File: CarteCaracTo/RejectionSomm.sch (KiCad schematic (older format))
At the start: 6 parts, among them U1 OPA4376

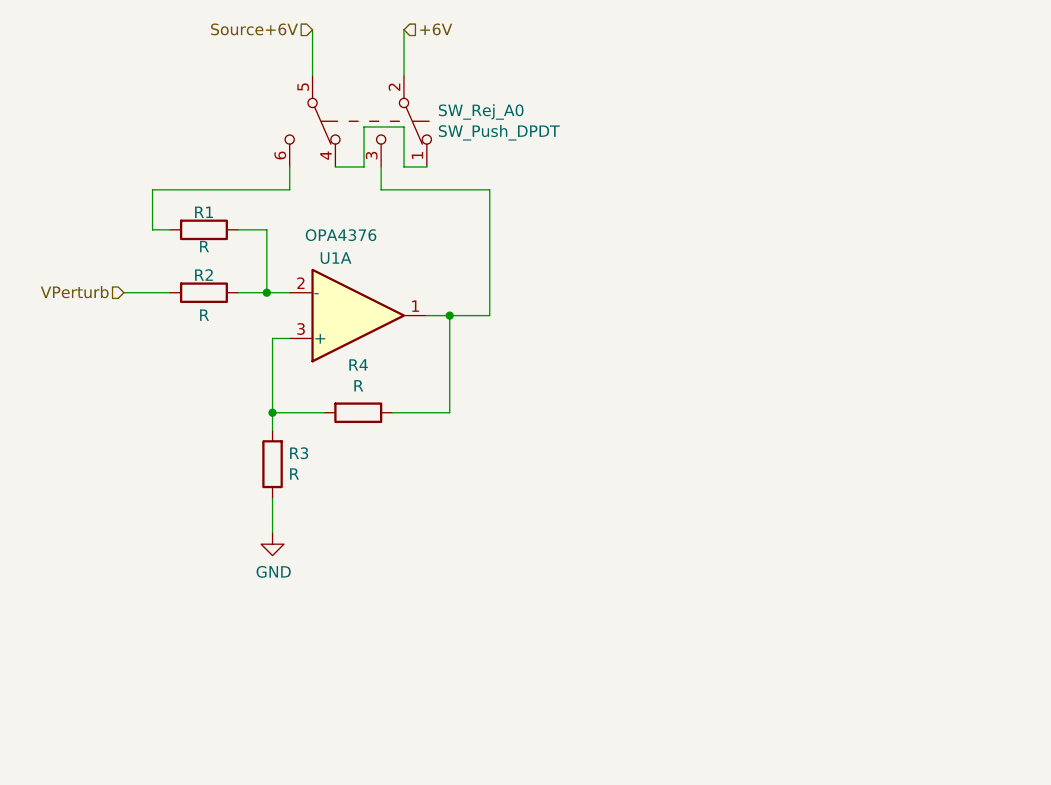
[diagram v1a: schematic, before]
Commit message: Routé, verif pre-envoie
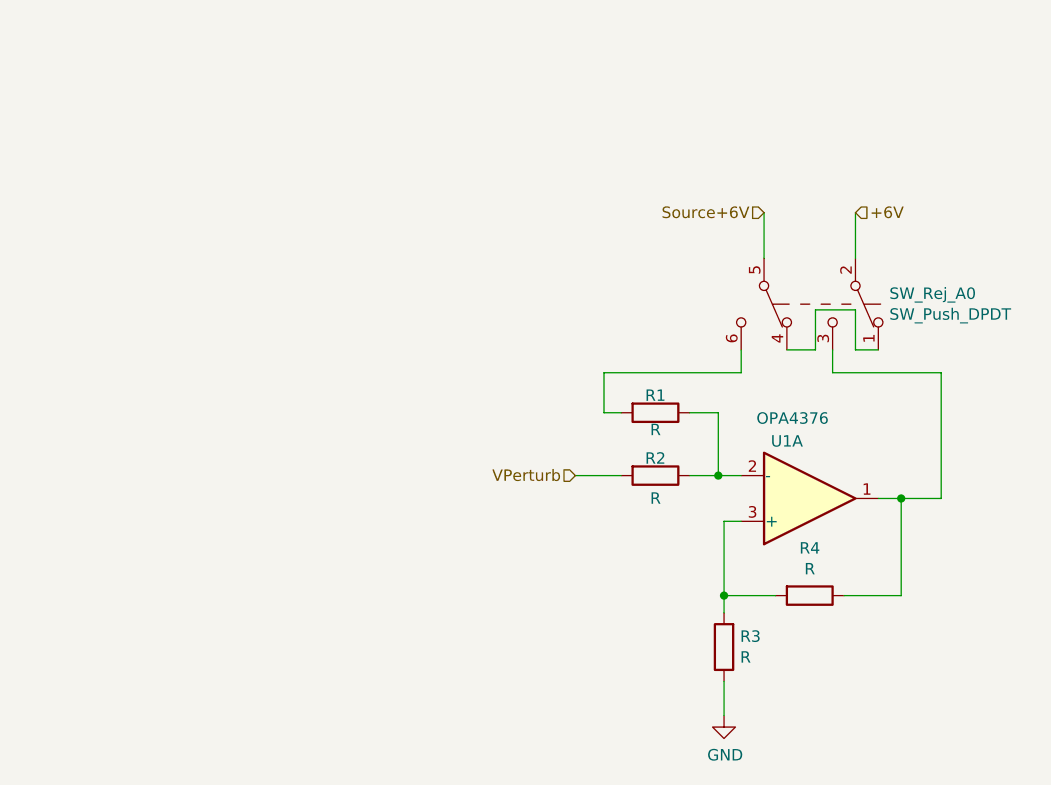
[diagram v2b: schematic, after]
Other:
- moved on the sheet: R1, R2, R3, R4, SW_Rej_A0, U1A
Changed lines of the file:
@@
 $Descr A4 11693 8268
 encoding utf-8
-Sheet 121 122
+Sheet 120 122
 Title ""
 Date ""
@@
 L Amplifier_Operational:OPA4376 U?
 U 1 1 61D78C60
-P 3450 3075
+P 5425 3875
 AR Path="/61D78C60" Ref="U?"  Part="1"
 AR Path="/61D6BED7/61D78C60" Ref="U1"  Part="1"
 AR Path="/61F56081/61D78C60" Ref="U1"  Part="2"
 AR Path="/61F9BC15/61D78C60" Ref="U1"  Part="3"
-F 0 "U1" H 3350 2825 50  0000 C CNN
-F 1 "OPA4376" H 3375 2725 50  0000 C CNN
-F 2 "Package_SO:SOIC-14_3.9x8.7mm_P1.27mm" H 3400 3175 50  0001 C CNN
-F 3 "http://www.ti.com/lit/ds/symlink/opa376.pdf" H 3500 3275 50  0001 C CNN
-	1    3450 3075
+F 0 "U1" H 5325 3625 50  0000 C CNN
+F 1 "OPA4376" H 5350 3525 50  0000 C CNN
+F 2 "Package_SO:SOIC-14_3.9x8.7mm_P1.27mm" H 5375 3975 50  0001 C CNN
+F 3 "http://www.ti.com/lit/ds/symlink/opa376.pdf" H 5475 4075 50  0001 C CNN
+	1    5425 3875
 	1    0    0    1
 $EndComp
@@
 L Device:R R?
 U 1 1 61D78C66
-P 2775 2700
+P 4750 3500
 AR Path="/61D78C66" Ref="R?"  Part="1"
 AR Path="/61D6BED7/61D78C66" Ref="R1"  Part="1"
 AR Path="/61F56081/61D78C66" Ref="R5"  Part="1"
 AR Path="/61F9BC15/61D78C66" Ref="R9"  Part="1"
-F 0 "R1" V 2700 2700 50  0000 C CNN
-F 1 "R" V 2850 2700 50  0000 C CNN
-F 2 "Resistor_SMD:R_0603_1608Metric_Pad1.05x0.95mm_HandSolder" V 2705 2700 50  0001 C CNN
-F 3 "~" H 2775 2700 50  0001 C CNN
-	1    2775 2700
+F 0 "R1" V 4675 3500 50  0000 C CNN
+F 1 "R" V 4825 3500 50  0000 C CNN
+F 2 "Resistor_SMD:R_0603_1608Metric_Pad1.05x0.95mm_HandSolder" V 4680 3500 50  0001 C CNN
+F 3 "~" H 4750 3500 50  0001 C CNN
+	1    4750 3500
 	0    1    1    0
 $EndComp
@@
 L Device:R R?
 U 1 1 61D78C6C
-P 2775 2975
+P 4750 3775
 AR Path="/61D78C6C" Ref="R?"  Part="1"
 AR Path="/61D6BED7/61D78C6C" Ref="R2"  Part="1"
 AR Path="/61F56081/61D78C6C" Ref="R6"  Part="1"
 AR Path="/61F9BC15/61D78C6C" Ref="R10"  Part="1"
-F 0 "R2" V 2700 2975 50  0000 C CNN
-F 1 "R" V 2875 2975 50  0000 C CNN
-F 2 "Resistor_SMD:R_0603_1608Metric_Pad1.05x0.95mm_HandSolder" V 2705 2975 50  0001 C CNN
-F 3 "~" H 2775 2975 50  0001 C CNN
-	1    2775 2975
+F 0 "R2" V 4675 3775 50  0000 C CNN
+F 1 "R" V 4850 3775 50  0000 C CNN
+F 2 "Resistor_SMD:R_0603_1608Metric_Pad1.05x0.95mm_HandSolder" V 4680 3775 50  0001 C CNN
+F 3 "~" H 4750 3775 50  0001 C CNN
+	1    4750 3775
 	0    1    1    0
 $EndComp
@@
 L Device:R R?
 U 1 1 61D78C72
-P 3075 3725
+P 5050 4525
 AR Path="/61D78C72" Ref="R?"  Part="1"
 AR Path="/61D6BED7/61D78C72" Ref="R3"  Part="1"
 AR Path="/61F56081/61D78C72" Ref="R7"  Part="1"
 AR Path="/61F9BC15/61D78C72" Ref="R11"  Part="1"
-F 0 "R3" H 3005 3679 50  0000 R CNN
-F 1 "R" H 3005 3770 50  0000 R CNN
-F 2 "Resistor_SMD:R_0603_1608Metric_Pad1.05x0.95mm_HandSolder" V 3005 3725 50  0001 C CNN
-F 3 "~" H 3075 3725 50  0001 C CNN
-	1    3075 3725
+F 0 "R3" H 4980 4479 50  0000 R CNN
+F 1 "R" H 4980 4570 50  0000 R CNN
+F 2 "Resistor_SMD:R_0603_1608Metric_Pad1.05x0.95mm_HandSolder" V 4980 4525 50  0001 C CNN
+F 3 "~" H 5050 4525 50  0001 C CNN
+	1    5050 4525
 	-1   0    0    1
 $EndComp
@@
 L Device:R R?
 U 1 1 61D78C78
-P 3450 3500
+P 5425 4300
 AR Path="/61D78C78" Ref="R?"  Part="1"
 AR Path="/61D6BED7/61D78C78" Ref="R4"  Part="1"
 AR Path="/61F56081/61D78C78" Ref="R8"  Part="1"
 AR Path="/61F9BC15/61D78C78" Ref="R12"  Part="1"
-F 0 "R4" V 3243 3500 50  0000 C CNN
-F 1 "R" V 3334 3500 50  0000 C CNN
-F 2 "Resistor_SMD:R_0603_1608Metric_Pad1.05x0.95mm_HandSolder" V 3380 3500 50  0001 C CNN
-F 3 "~" H 3450 3500 50  0001 C CNN
-	1    3450 3500
+F 0 "R4" V 5218 4300 50  0000 C CNN
+F 1 "R" V 5309 4300 50  0000 C CNN
+F 2 "Resistor_SMD:R_0603_1608Metric_Pad1.05x0.95mm_HandSolder" V 5355 4300 50  0001 C CNN
+F 3 "~" H 5425 4300 50  0001 C CNN
+	1    5425 4300
 	0    1    1    0
 $EndComp
 Wire Wire Line
-	2925 2700 3050 2700
+	4900 3500 5025 3500
 Wire Wire Line
-	3050 2700 3050 2975
+	5025 3500 5025 3775
 Wire Wire Line
-	3050 2975 3150 2975
+	5025 3775 5125 3775
 Wire Wire Line
-	2925 2975 3050 2975
-Connection ~ 3050 2975
+	4900 3775 5025 3775
+Connection ~ 5025 3775
 Wire Wire Line
-	3650 2025 3650 1825
+	5625 2825 5625 2625
 Wire Wire Line
-	2625 2975 2425 2975
+	4600 3775 4400 3775
 Wire Wire Line
-	3150 3175 3075 3175
+	5125 3975 5050 3975
 Wire Wire Line
-	3075 3175 3075 3500
+	5050 3975 5050 4300
 Wire Wire Line
-	3300 3500 3075 3500
-Connection ~ 3075 3500
+	5275 4300 5050 4300
+Connection ~ 5050 4300
 Wire Wire Line
-	3075 3500 3075 3575
+	5050 4300 5050 4375
 Wire Wire Line
-	3600 3500 3850 3500
+	5575 4300 5825 4300
 Wire Wire Line
-	3850 3500 3850 3075
+	5825 4300 5825 3875
 Wire Wire Line
-	3850 3075 3750 3075
+	5825 3875 5725 3875
 Wire Wire Line
-	3850 3075 4025 3075
-Connection ~ 3850 3075
+	5825 3875 6000 3875
+Connection ~ 5825 3875
 Wire Wire Line
-	3075 3875 3075 4025
+	5050 4675 5050 4825
 $Comp
 L power:GND #PWR?
 U 1 1 61D78C90
-P 3075 4025
+P 5050 4825
 AR Path="/61D78C90" Ref="#PWR?"  Part="1"
 AR Path="/61D6BED7/61D78C90" Ref="#PWR09"  Part="1"
 AR Path="/61F56081/61D78C90" Ref="#PWR010"  Part="1"
 AR Path="/61F9BC15/61D78C90" Ref="#PWR011"  Part="1"
-F 0 "#PWR011" H 3075 3775 50  0001 C CNN
-F 1 "GND" H 3080 3852 50  0000 C CNN
-F 2 "" H 3075 4025 50  0001 C CNN
-F 3 "" H 3075 4025 50  0001 C CNN
-	1    3075 4025
+F 0 "#PWR011" H 5050 4575 50  0001 C CNN
+F 1 "GND" H 5055 4652 50  0000 C CNN
+F 2 "" H 5050 4825 50  0001 C CNN
+F 3 "" H 5050 4825 50  0001 C CNN
+	1    5050 4825
 	1    0    0    -1
 $EndComp
@@
 L Switch:SW_Push_DPDT SW?
 U 1 1 61D78C98
-P 3450 2225
+P 5425 3025
 AR Path="/61D78C98" Ref="SW?"  Part="1"
 AR Path="/61D6BED7/61D78C98" Ref="SW_Rej_A0"  Part="1"
 AR Path="/61F56081/61D78C98" Ref="SW_RegB0"  Part="1"
 AR Path="/61F9BC15/61D78C98" Ref="SW_Rej_C0"  Part="1"
-F 0 "SW_Rej_A0" V 3404 2573 50  0000 L CNN
-F 1 "SW_Push_DPDT" V 3495 2573 50  0000 L CNN
-F 2 "LibPersoNadj:SW_DPDT_B22AP_NKK" H 3450 2425 50  0001 C CNN
-F 3 "~" H 3450 2425 50  0001 C CNN
-	1    3450 2225
+F 0 "SW_Rej_A0" V 5379 3373 50  0000 L CNN
+F 1 "SW_Push_DPDT" V 5470 3373 50  0000 L CNN
+F 2 "LibPersoNadj:SW_DPDT_B22AP_NKK" H 5425 3225 50  0001 C CNN
+F 3 "~" H 5425 3225 50  0001 C CNN
+	1    5425 3025
 	0    1    1    0
 $EndComp
 Wire Wire Line
-	3250 2025 3250 1825
+	5225 2825 5225 2625
 Wire Wire Line
-	3350 2425 3475 2425
+	5325 3225 5450 3225
 Wire Wire Line
-	3475 2425 3475 2250
+	5450 3225 5450 3050
 Wire Wire Line
-	3475 2250 3650 2250
+	5450 3050 5625 3050
 Wire Wire Line
-	3650 2250 3650 2425
+	5625 3050 5625 3225
 Wire Wire Line
-	3650 2425 3750 2425
+	5625 3225 5725 3225
 Wire Wire Line
-	2550 2700 2625 2700
+	4525 3500 4600 3500
 Wire Wire Line
-	3550 2425 3550 2525
+	5525 3225 5525 3325
 Wire Wire Line
-	3550 2525 4025 2525
+	5525 3325 6000 3325
 Wire Wire Line
-	4025 2525 4025 3075
+	6000 3325 6000 3875
 Wire Wire Line
-	2550 2525 3150 2525
+	4525 3325 5125 3325
 Wire Wire Line
-	3150 2525 3150 2425
+	5125 3325 5125 3225
 Wire Wire Line
-	2550 2525 2550 2700
-Text HLabel 3250 1825 0    50   Input ~ 0
+	4525 3325 4525 3500
+Text HLabel 5225 2625 0    50   Input ~ 0
 Source+6V
-Text HLabel 3650 1825 2    50   Input ~ 0
+Text HLabel 5625 2625 2    50   Input ~ 0
 +6V
-Text HLabel 2425 2975 0    50   Input ~ 0
+Text HLabel 4400 3775 0    50   Input ~ 0
 VPerturb
 $EndSCHEMATC
